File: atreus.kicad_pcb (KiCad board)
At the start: 2 copper layers, 232 x 90 mm, 99 parts, among them U1 ATmega32U4-AU, Y1 Crystal_GND24_Small

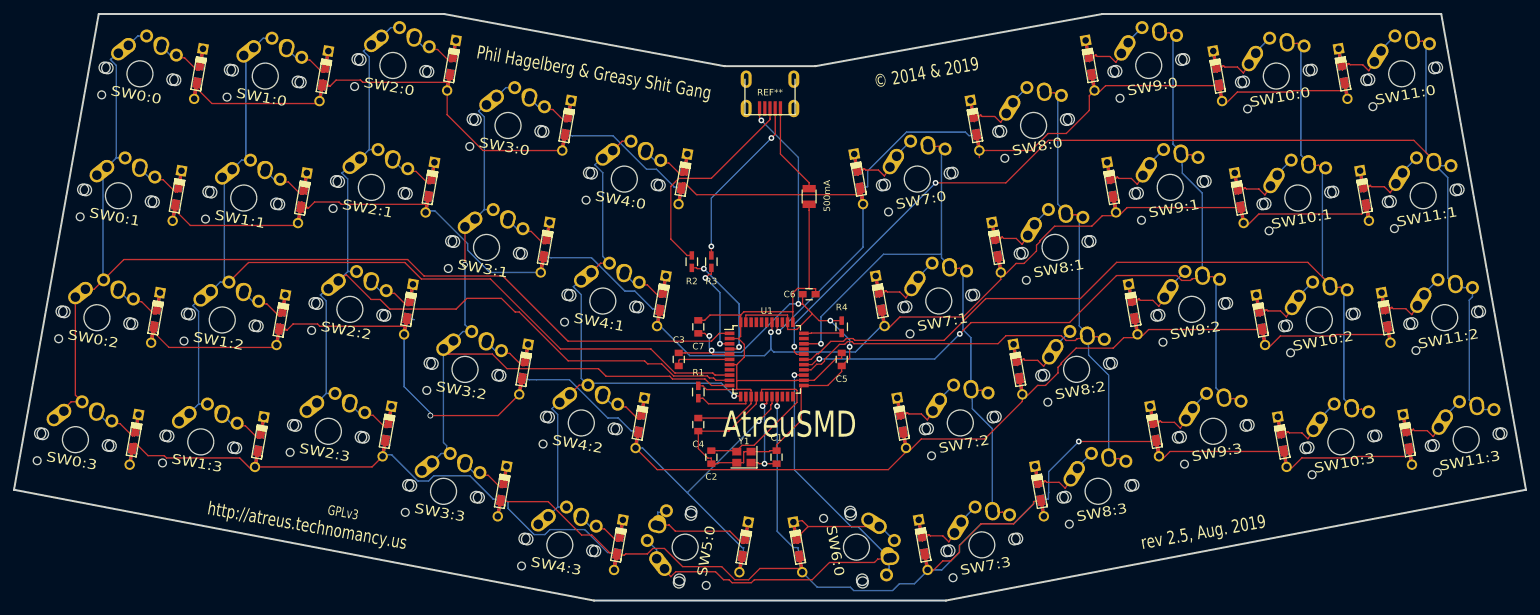
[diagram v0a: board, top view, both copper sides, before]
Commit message: manually traced the thing.
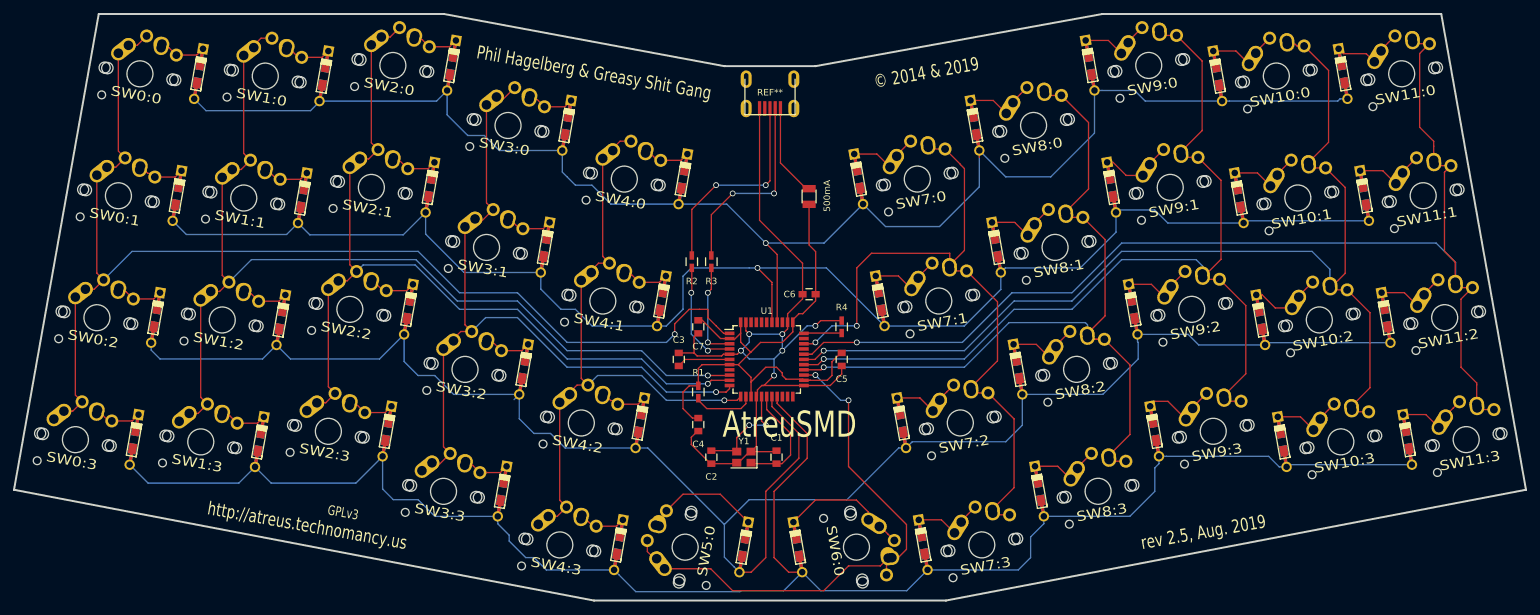
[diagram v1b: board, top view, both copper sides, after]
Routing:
- net GND: track 143.0 -> 0.00 mm, vias 6 -> 0
- net 59: track 0.00 -> 131.0 mm, vias 0 -> 6
- net +5V: track 89.8 -> 0.00 mm
- net 62: track 0.00 -> 86.7 mm
- net N-row-3: track 349.8 -> 265.4 mm, vias 2 -> 0
- net N-row-2: track 332.7 -> 272.8 mm, vias 2 -> 0
- net N-row-0: track 288.8 -> 230.0 mm
- net N-row-1: track 272.9 -> 229.3 mm
- net 66: track 0.00 -> 32.0 mm, vias 0 -> 2
- net Net-C2-Pad1: track 24.8 -> 0.00 mm
- net D+: track 33.5 -> 15.1 mm, vias 0 -> 2
- net Net-R2-Pad1: track 17.7 -> 0.00 mm, vias 2 -> 0
- net 65: track 0.00 -> 17.2 mm, vias 0 -> 2
- net 58: track 0.00 -> 17.2 mm
- net 60: track 0.00 -> 16.0 mm, vias 0 -> 2
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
